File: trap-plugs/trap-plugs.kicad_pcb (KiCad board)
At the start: 2 copper layers, 58 x 29 mm, 7 parts, among them J2 JCON_M16_04Pin, J4 Conn_01x08, J5 JCON_M16_2+4Pin, J6 JCON_M16_2+4Pin

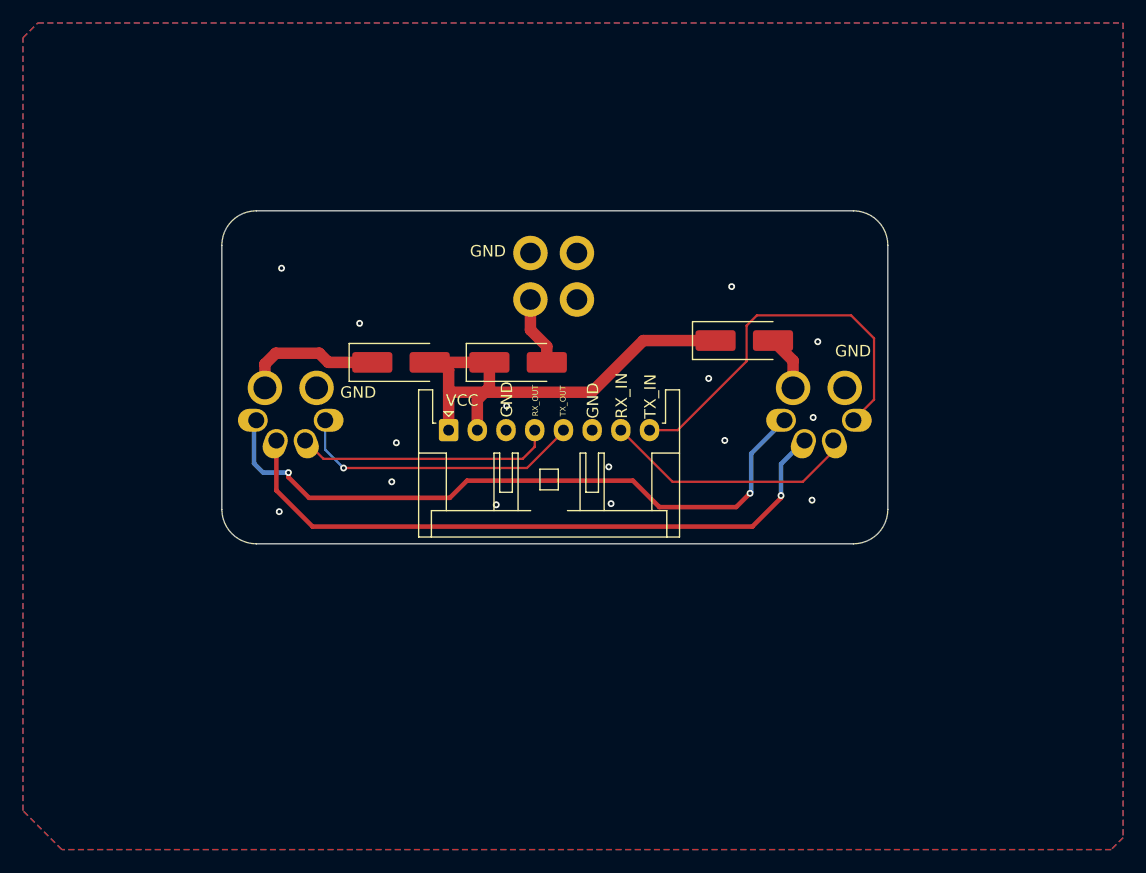
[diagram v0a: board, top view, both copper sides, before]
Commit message: WIP
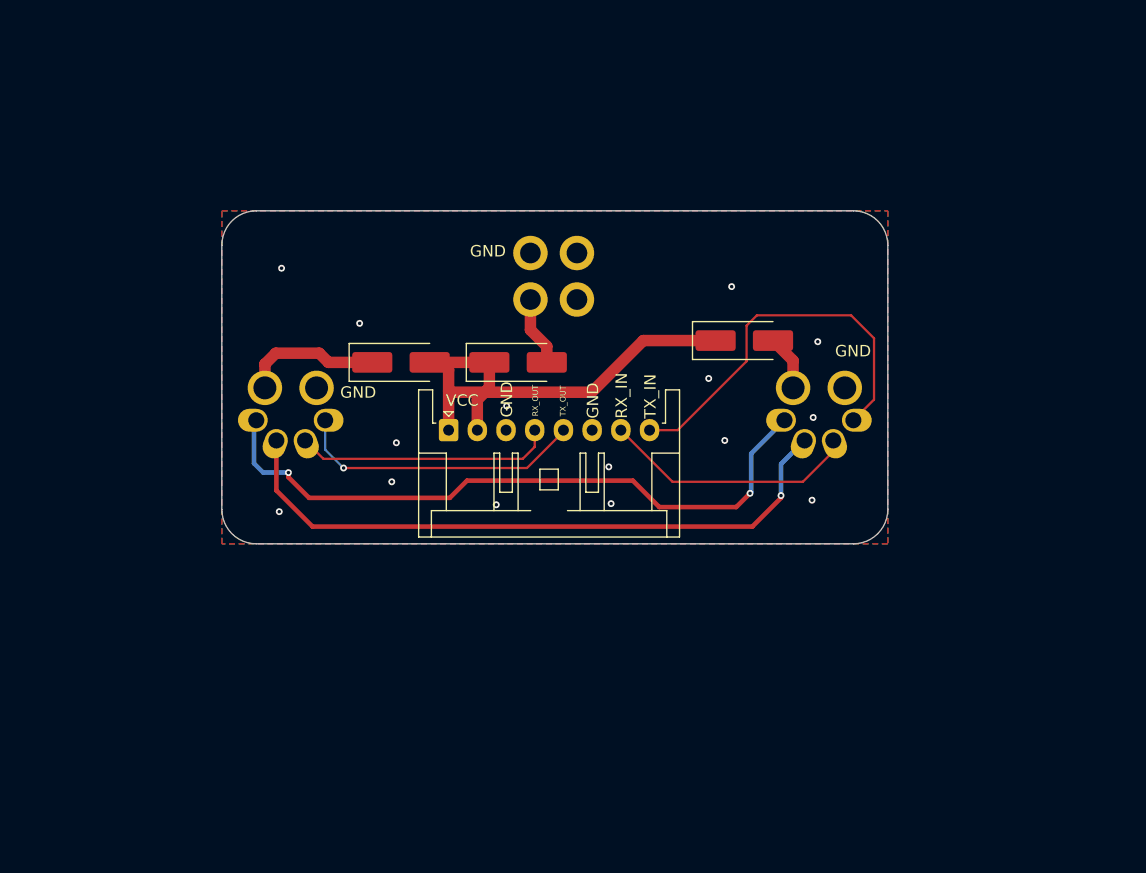
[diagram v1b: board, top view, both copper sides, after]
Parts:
- added REF**: Tab, kikit:Tab, F.Cu at (169.0, 97.5)
- added REF**: Tab, kikit:Tab, F.Cu at (129.0, 97.5)
- added REF**: Tab, kikit:Tab, F.Cu at (130.0, 67.5)
- added REF**: Tab, kikit:Tab, F.Cu at (120.5, 76.0)
- added REF**: Tab, kikit:Tab, F.Cu at (170.0, 67.5)
- added REF**: Tab, kikit:Tab, F.Cu at (149.0, 97.5)
- added REF**: Tab, kikit:Tab, F.Cu at (180.6, 76.0)
- added REF**: Tab, kikit:Tab, F.Cu at (150.0, 67.5)
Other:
- copper layers 2 -> 4
